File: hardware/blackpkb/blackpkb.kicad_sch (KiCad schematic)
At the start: 30 parts, among them SW1 SW_Push_45deg, SW10 SW_Push_45deg, SW11 SW_Push_45deg, SW12 SW_Push_45deg, SW13 RotaryEncoder_Switch, SW2 SW_Push_45deg, SW3 SW_Push_45deg, SW4 SW_Push_45deg, SW5 SW_Push_45deg, SW6 SW_Push_45deg, SW7 SW_Push_45deg, SW8 SW_Push_45deg, SW9 SW_Push_45deg, U1 YAAJ_WeAct_BlackPill_Part_Lik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

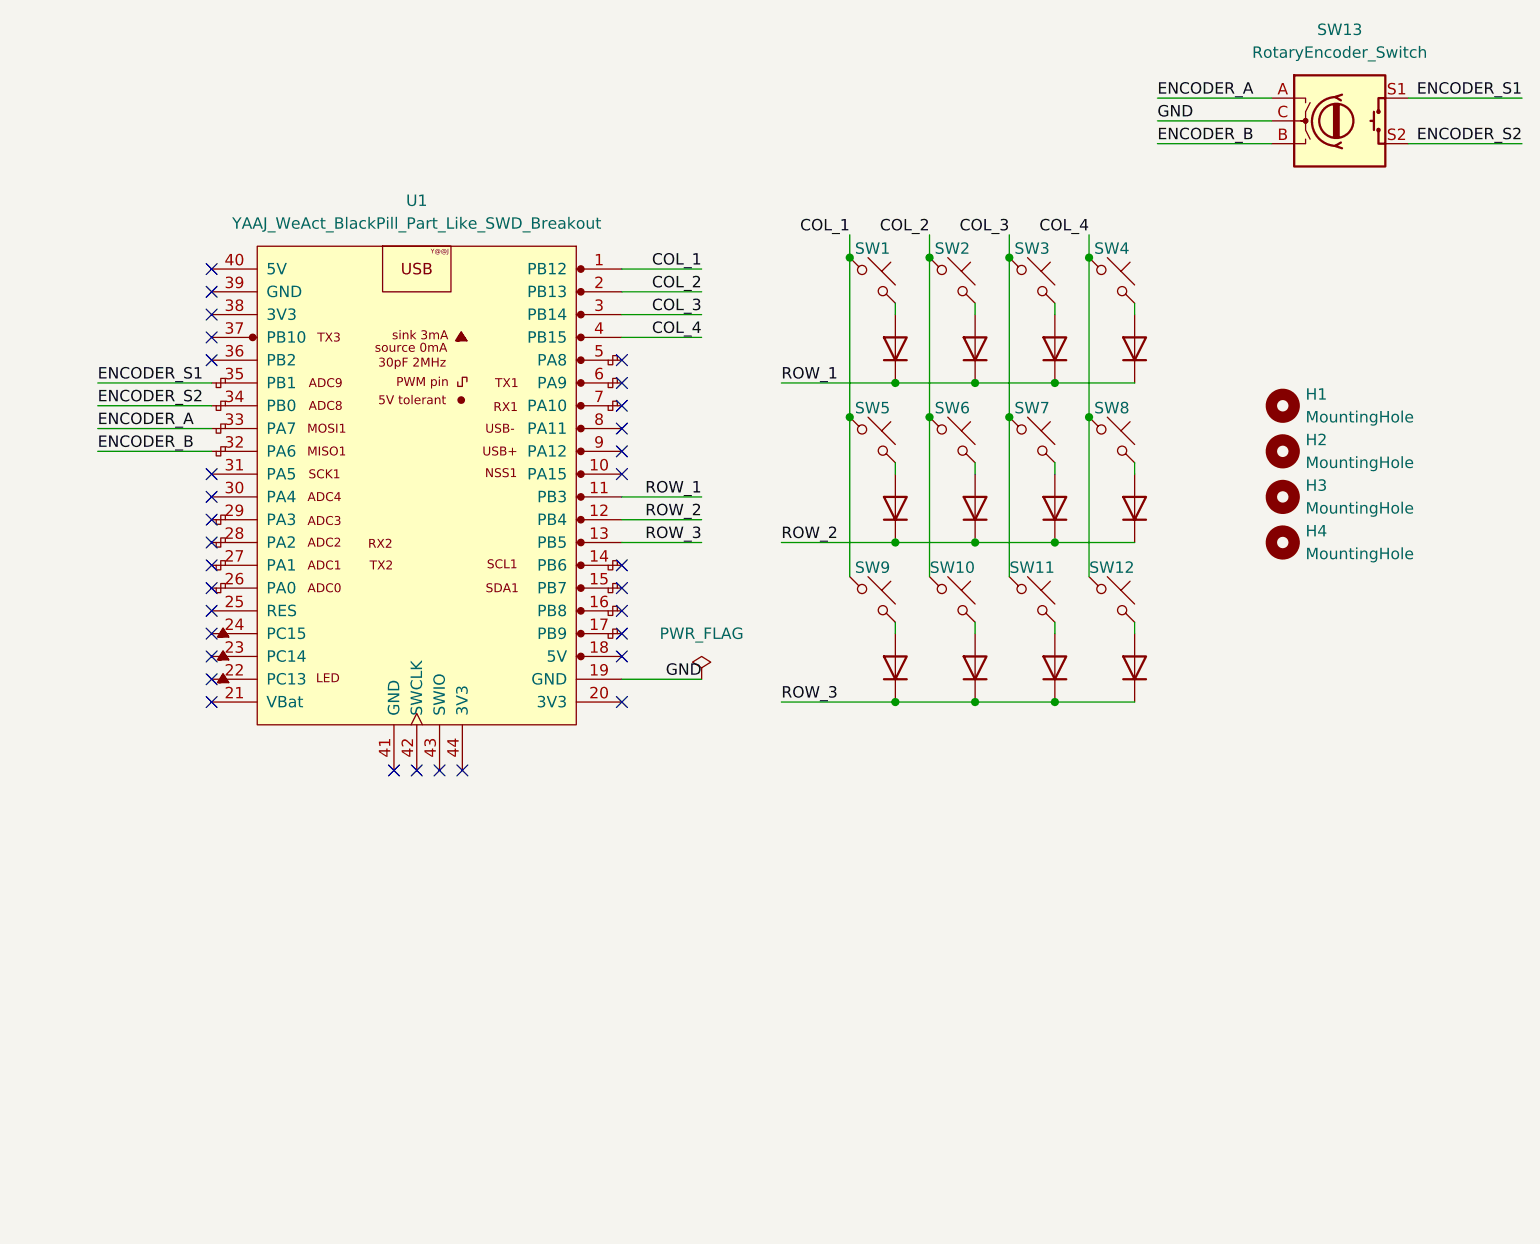
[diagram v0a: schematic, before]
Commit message: section the schematic. Add infomations, remove redundant files
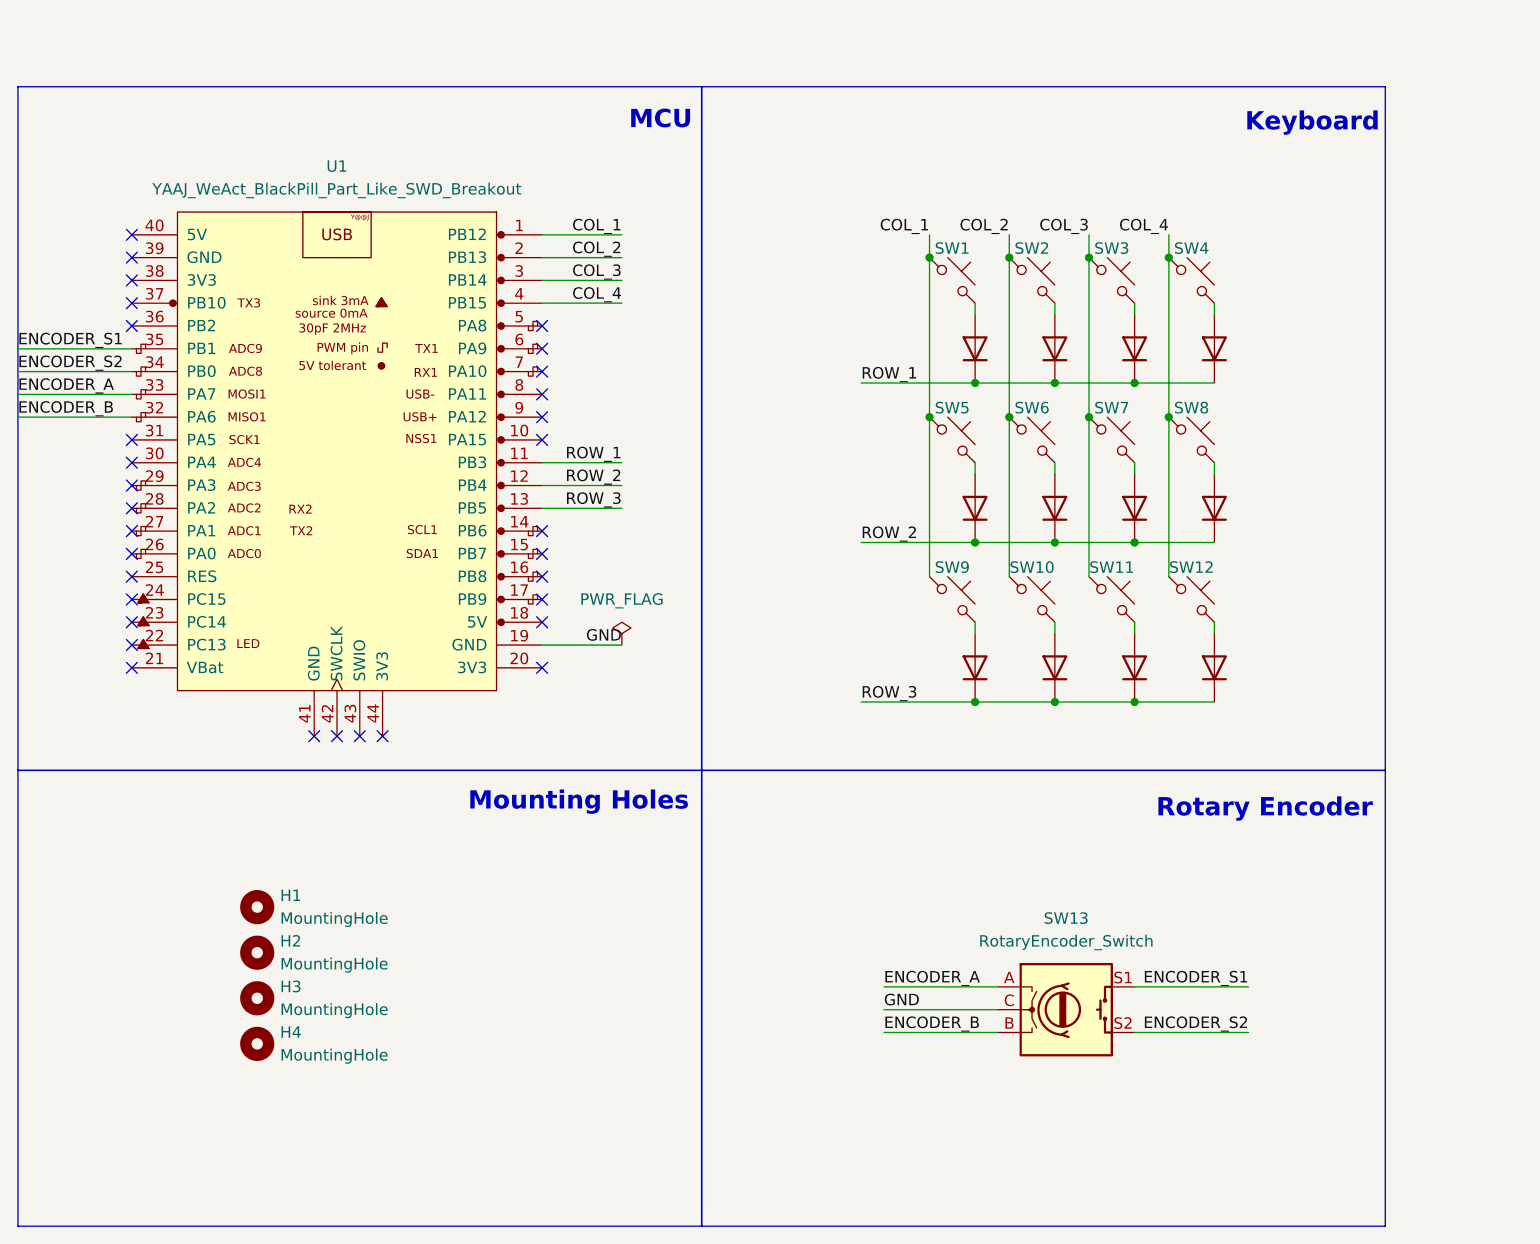
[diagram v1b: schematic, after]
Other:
- note added: "Keyboard"
- note added: "MCU"
- note added: "Mounting Holes"
- note added: "Rotary Encoder"
- company: (none) -> author - alcato
- title: (none) -> blackpkb
- moved on the sheet: H1, H2, H3, H4, SW1, SW10, SW11, SW12, SW13, SW2, SW3, SW4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
